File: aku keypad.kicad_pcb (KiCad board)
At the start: 2 copper layers, 47.6 x 46 mm, 19 parts, among them J1 USB_C_Receptacle_USB2.0, SW1 SW_Push, SW2 MX_SW_HS, SW3 MX_SW_HS, U1 SRV05-4, U2 ATmega32U2-M, Y1 Crystal_GND24_Small

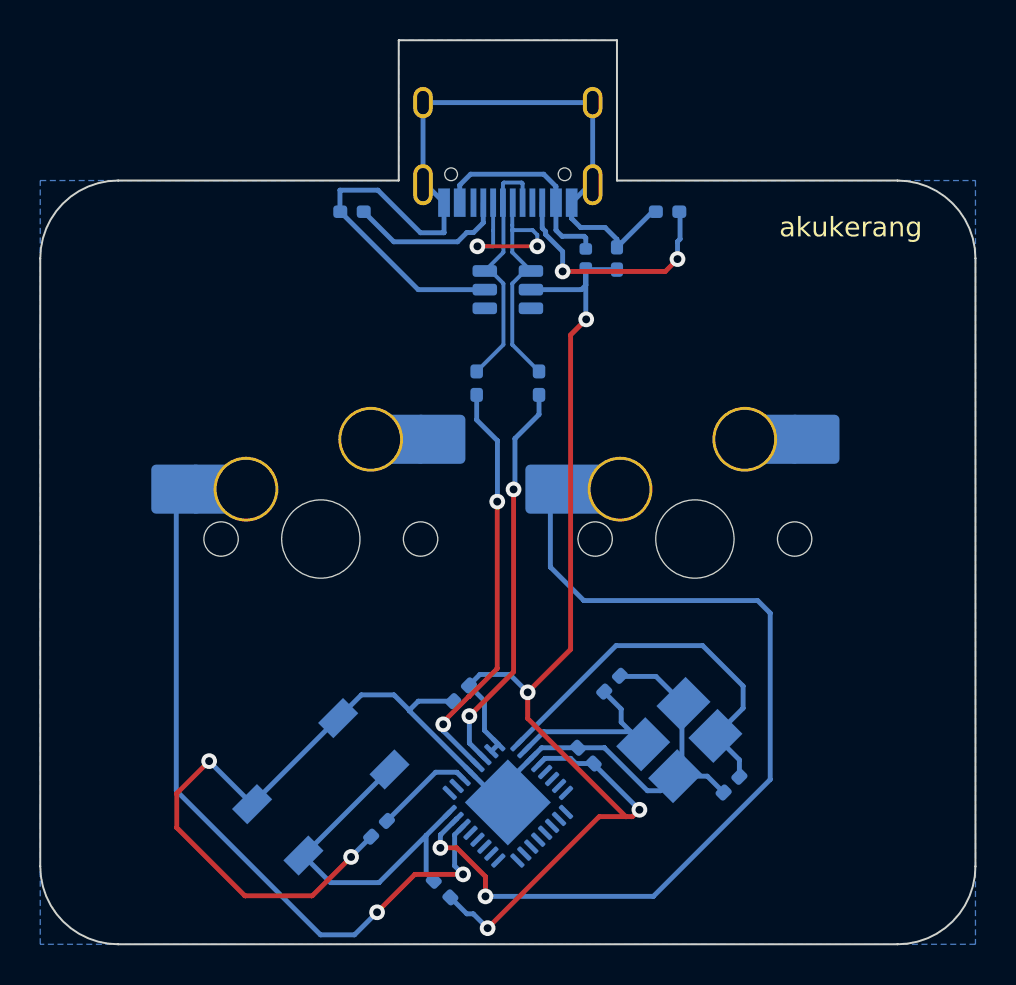
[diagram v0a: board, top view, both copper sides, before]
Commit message: Added front ground fill
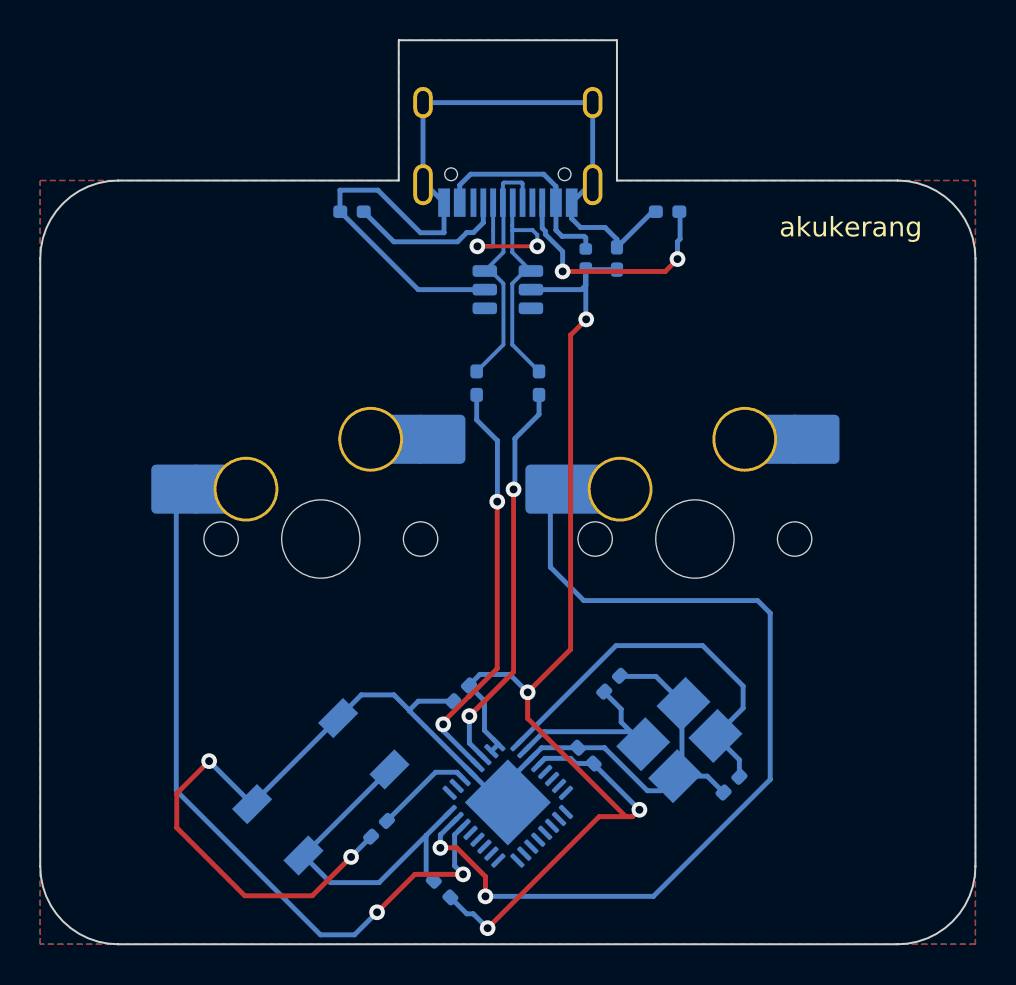
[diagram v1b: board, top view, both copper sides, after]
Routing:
- added copper zone on F.Cu, net GND
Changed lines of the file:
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@@
   (segment (start 47.7525 78.10125) (end 48.9025 76.95125) (width 0.25) (layer "B.Cu") (net 38))
   (segment (start 53.308597 72.549493) (end 52.851574 73.006516) (width 0.25) (layer "B.Cu") (net 38))
+  (zone (net 1) (net_name "GND") (layer "F.Cu") (hatch edge 0.508)
+    (connect_pads (clearance 0.508))
+    (min_thickness 0.254) (filled_areas_thickness no)
+    (fill yes (thermal_gap 0.508) (thermal_bridge_width 0.508))
+    (polygon
+      (pts
+        (xy 61.11875 39.6875)
+        (xy 79.375 39.6875)
+        (xy 79.375 78.58125)
+        (xy 31.75 78.58125)
+        (xy 31.75 39.6875)
+        (xy 50.00625 39.6875)
+        (xy 50.00625 32.54375)
+        (xy 61.11875 32.54375)
+      )
+    )
+  )
   (zone (net 1) (net_name "GND") (layer "B.Cu") (hatch edge 0.508)
     (connect_pads yes (clearance 0.508))
